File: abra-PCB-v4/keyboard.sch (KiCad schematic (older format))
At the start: 295 parts, among them J2 Conn_01x04, P1 TC2030-AVR, Q1 Q_NPN_BCE, SW1 Rotary_Encoder_Switch, SW2 SW_Push, U1 ATmega32U4-AU, U2 PRTR5V0U2X, Y1 16MHz

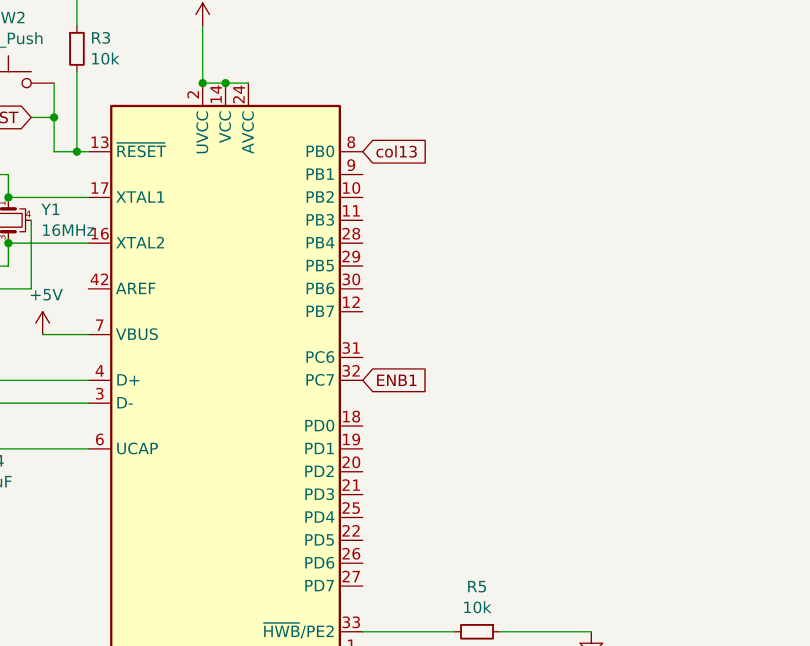
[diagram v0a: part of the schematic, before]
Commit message: routing updates
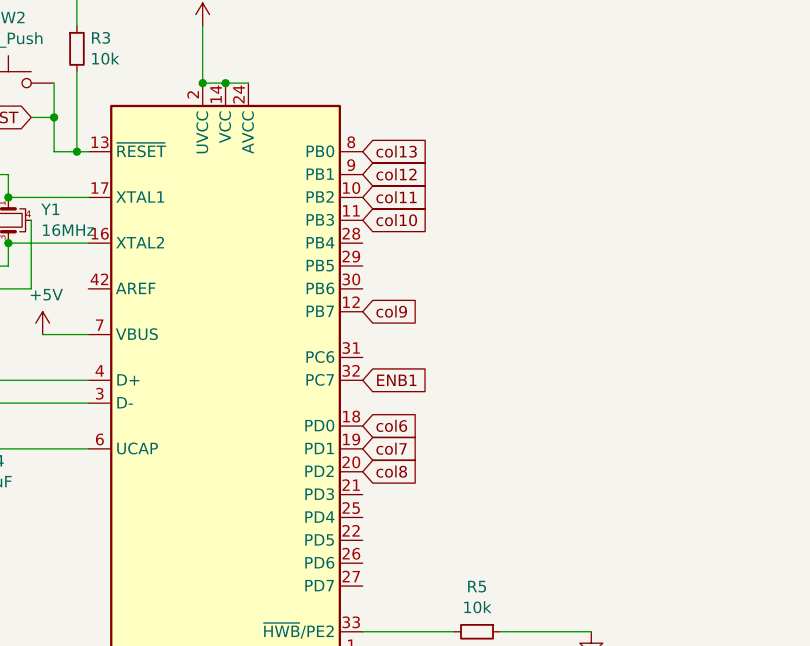
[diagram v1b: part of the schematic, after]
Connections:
- net col10: now also U1.11 (PB3)
- net col11: now also U1.10 (PB2)
- net col12: now also U1.9 (PB1)
- net col6: now also U1.18 (PD0)
- net col7: now also U1.19 (PD1)
- net col8: now also U1.20 (PD2)
- net col9: now also U1.12 (PB7)
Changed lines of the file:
@@
 	6700 4500 7100 4500
-$Comp
-L keyboard-rescue:ATmega32U4-AU-MCU_Microchip_ATmega U1
-U 1 1 5F1D63B5
-P 2350 6700
-F 0 "U1" H 2350 4811 50  0000 C CNN
-F 1 "ATmega32U4-AU" H 2350 4720 50  0000 C CNN
-F 2 "Package_QFP:TQFP-44_10x10mm_P0.8mm" H 2350 6700 50  0001 C CIN
-F 3 "http://ww1.microchip.com/downloads/en/DeviceDoc/Atmel-7766-8-bit-AVR-ATmega16U4-32U4_Datasheet.pdf" H 2350 6700 50  0001 C CNN
-	1    2350 6700
-	1    0    0    -1
-$EndComp
 $Comp
 L power:GND #PWR0101
@@
 Text GLabel 2950 5200 2    50   Input ~ 0
 col13
+Text GLabel 2950 5300 2    50   Input ~ 0
+col12
+Text GLabel 2950 5400 2    50   Input ~ 0
+col11
+Text GLabel 2950 5500 2    50   Input ~ 0
+col10
+$Comp
+L keyboard-rescue:ATmega32U4-AU-MCU_Microchip_ATmega U1
+U 1 1 5F1D63B5
+P 2350 6700
+F 0 "U1" H 2350 4811 50  0000 C CNN
+F 1 "ATmega32U4-AU" H 2350 4720 50  0000 C CNN
+F 2 "Package_QFP:TQFP-44_10x10mm_P0.8mm" H 2350 6700 50  0001 C CIN
+F 3 "http://ww1.microchip.com/downloads/en/DeviceDoc/Atmel-7766-8-bit-AVR-ATmega16U4-32U4_Datasheet.pdf" H 2350 6700 50  0001 C CNN
+	1    2350 6700
+	1    0    0    -1
+$EndComp
+Text GLabel 2950 5900 2    50   Input ~ 0
+col9
+Text GLabel 2950 6400 2    50   Input ~ 0
+col6
+Text GLabel 2950 6500 2    50   Input ~ 0
+col7
+Text GLabel 2950 6600 2    50   Input ~ 0
+col8
 $EndSCHEMATC

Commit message: routing updates
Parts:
- removed P1: TC2030-AVR, Keebio-Parts:Header-6-Pin-ZigZag, symbol keyboard-rescue:TC2030-AVR-keebio
- SW2: footprint random-keyboard-parts:Reset_Pretty -> Keebio-Parts:SW_SPST_3x3
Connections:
- net GND: now also SW1.C
- net row0: now also U1.21 (PD3)
- net row1: now also U1.22 (PD5)
- net row3: now also U1.25 (PD4)
- net row4: now also U1.31 (PC6)
- net row5: now also U1.30 (PB6)
- net ENA: now reaches U1.28 (PB4)
- net ENA: now also SW1.A
- net ENB: now reaches U1.29 (PB5)
- net ENB: now also SW1.B
- net RST: no longer names the net of R3.2, SW2.2, U1.13 (~RESET)
- no-connect marks 2 -> 3
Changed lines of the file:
@@
 EESchema Schematic File Version 4
+LIBS:keyboard-cache
 EELAYER 30 0
 EELAYER END
@@
 	1    0    0    -1
 $EndComp
-Wire Wire Line
-	22000 8700 22100 8700
-Wire Wire Line
-	22000 8500 22100 8500
-Text GLabel 22100 8700 2    50   Input ~ 0
+Text GLabel 22000 8700 2    50   Input ~ 0
 ENB2
-Text GLabel 22100 8500 2    50   Input ~ 0
+Text GLabel 22000 8500 2    50   Input ~ 0
 ENB1
 Text GLabel 21300 1300 0    50   Input ~ 0
@@
 F 0 "SW2" H 1400 5185 50  0000 C CNN
 F 1 "SW_Push" H 1400 5094 50  0000 C CNN
-F 2 "random-keyboard-parts:Reset_Pretty" H 1400 5100 50  0001 C CNN
+F 2 "Keebio-Parts:SW_SPST_3x3" H 1400 5100 50  0001 C CNN
 F 3 "~" H 1400 5100 50  0001 C CNN
 	1    1400 4900
@@
 $EndComp
 Wire Wire Line
-	1600 4900 1600 5050
-Wire Wire Line
 	1200 4900 950  4900
 $Comp
@@
 Connection ~ 19150 5450
 Connection ~ 19150 6450
-Text GLabel 2850 3400 0    50   Input ~ 0
-MISO
-Text GLabel 2850 3500 0    50   Input ~ 0
-SCK
-Text GLabel 2850 3600 0    50   Input ~ 0
-RST
-Text GLabel 3550 3500 2    50   Input ~ 0
-MOSI
-$Comp
-L power:GND #PWR0120
-U 1 1 6269E757
-P 3550 3600
-F 0 "#PWR0120" H 3550 3350 50  0001 C CNN
-F 1 "GND" H 3555 3427 50  0000 C CNN
-F 2 "" H 3550 3600 50  0001 C CNN
-F 3 "" H 3550 3600 50  0001 C CNN
-	1    3550 3600
-	1    0    0    -1
-$EndComp
-$Comp
-L power:+5V #PWR0121
-U 1 1 626A0384
-P 3550 3400
-F 0 "#PWR0121" H 3550 3250 50  0001 C CNN
-F 1 "+5V" H 3565 3573 50  0000 C CNN
-F 2 "" H 3550 3400 50  0001 C CNN
-F 3 "" H 3550 3400 50  0001 C CNN
-	1    3550 3400
-	1    0    0    -1
-$EndComp
-Text GLabel 1500 5050 0    50   Input ~ 0
-RST
-Wire Wire Line
-	1500 5050 1600 5050
-Connection ~ 1600 5050
-Wire Wire Line
-	1600 5050 1600 5200
-$Comp
-L keyboard-rescue:TC2030-AVR-keebio P1
-U 1 1 5F2CE766
-P 3200 3500
-F 0 "P1" H 3200 3792 40  0000 C CNN
-F 1 "TC2030-AVR" H 3200 3716 40  0000 C CNN
-F 2 "Keebio-Parts:Header-6-Pin-ZigZag" H 3200 3500 50  0001 C CNN
-F 3 "" H 3200 3500 50  0001 C CNN
-	1    3200 3500
-	1    0    0    -1
-$EndComp
 Wire Wire Line
 	3650 14900 3650 15000
@@
 Text GLabel 2950 6600 2    50   Input ~ 0
 col8
+NoConn ~ 1750 5800
+Text GLabel 2950 6700 2    50   Input ~ 0
+row0
+Wire Wire Line
+	1600 4900 1600 5200
+Text GLabel 2950 6900 2    50   Input ~ 0
+row1
+Text GLabel 2950 6800 2    50   Input ~ 0
+row3
+Text GLabel 2950 6100 2    50   Input ~ 0
+row4
+Text GLabel 2950 5800 2    50   Input ~ 0
+row5
+Text GLabel 21400 8500 0    50   Input ~ 0
+ENA
+Text GLabel 21400 8700 0    50   Input ~ 0
+ENB
+Wire Wire Line
+	21400 8600 21100 8600
+$Comp
+L power:GND #PWR0120
+U 1 1 5FBF5950
+P 21100 8600
+F 0 "#PWR0120" H 21100 8350 50  0001 C CNN
+F 1 "GND" H 21105 8427 50  0000 C CNN
+F 2 "" H 21100 8600 50  0001 C CNN
+F 3 "" H 21100 8600 50  0001 C CNN
+	1    21100 8600
+	1    0    0    -1
+$EndComp
+Text GLabel 2950 5600 2    50   Input ~ 0
+ENA
+Text GLabel 2950 5700 2    50   Input ~ 0
+ENB
 $EndSCHEMATC
